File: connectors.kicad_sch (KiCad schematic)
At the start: 4 parts, among them J1 UPT-08-01-01-L-RA, J2 UPT-08-01-01-L-RA, J3 Screw_Terminal_01x02, J4 Conn_01x06

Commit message: Minor fixes
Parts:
- removed J1, J2: UPT-08-01-01-L-RA, UPT080101LRA, symbol 8pin_good:UPT-08-01-01-L-RA
- added J1, J2: UPT-08-01-01-L-RA, UPT080101LRA, symbol UPT-08-01-01-L-RA:UPT-08-01-01-L-RA
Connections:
- net OUT1_0: now also J2.C1, J2.C2, J2.C3, J2.C4, J2.C5, J2.C6
- net OUT1_1: now also J2.B1, J2.B2, J2.B3, J2.B4, J2.B5, J2.B6
- net OUT1_2: now also J2.A1, J2.A2, J2.A3, J2.A4, J2.A5, J2.A6
- net OUT1_3: now also J2.D1, J2.D2, J2.D3, J2.D4, J2.D5, J2.D6
- net OUT2_0: now also J2.H1, J2.H2, J2.H3, J2.H4, J2.H5, J2.H6
- net OUT2_1: now also J2.G1, J2.G2, J2.G3, J2.G4, J2.G5, J2.G6
- net OUT2_2: now also J2.F1, J2.F2, J2.F3, J2.F4, J2.F5, J2.F6
- net OUT2_3: now also J2.E1, J2.E2, J2.E3, J2.E4, J2.E5, J2.E6
- net OUT3_0: now also J1.D1, J1.D2, J1.D3, J1.D4, J1.D5, J1.D6
- net OUT3_1: now also J1.C1, J1.C2, J1.C3, J1.C4, J1.C5, J1.C6
- net OUT3_2: now also J1.B1, J1.B2, J1.B3, J1.B4, J1.B5, J1.B6
- net OUT3_3: now also J1.A1, J1.A2, J1.A3, J1.A4, J1.A5, J1.A6
- net OUT4_0: now also J1.H1, J1.H2, J1.H3, J1.H4, J1.H5, J1.H6
- net OUT4_1: now also J1.G1, J1.G2, J1.G3, J1.G4, J1.G5, J1.G6
- net OUT4_2: now also J1.F1, J1.F2, J1.F3, J1.F4, J1.F5, J1.F6
- net OUT4_3: now also J1.E1, J1.E2, J1.E3, J1.E4, J1.E5, J1.E6

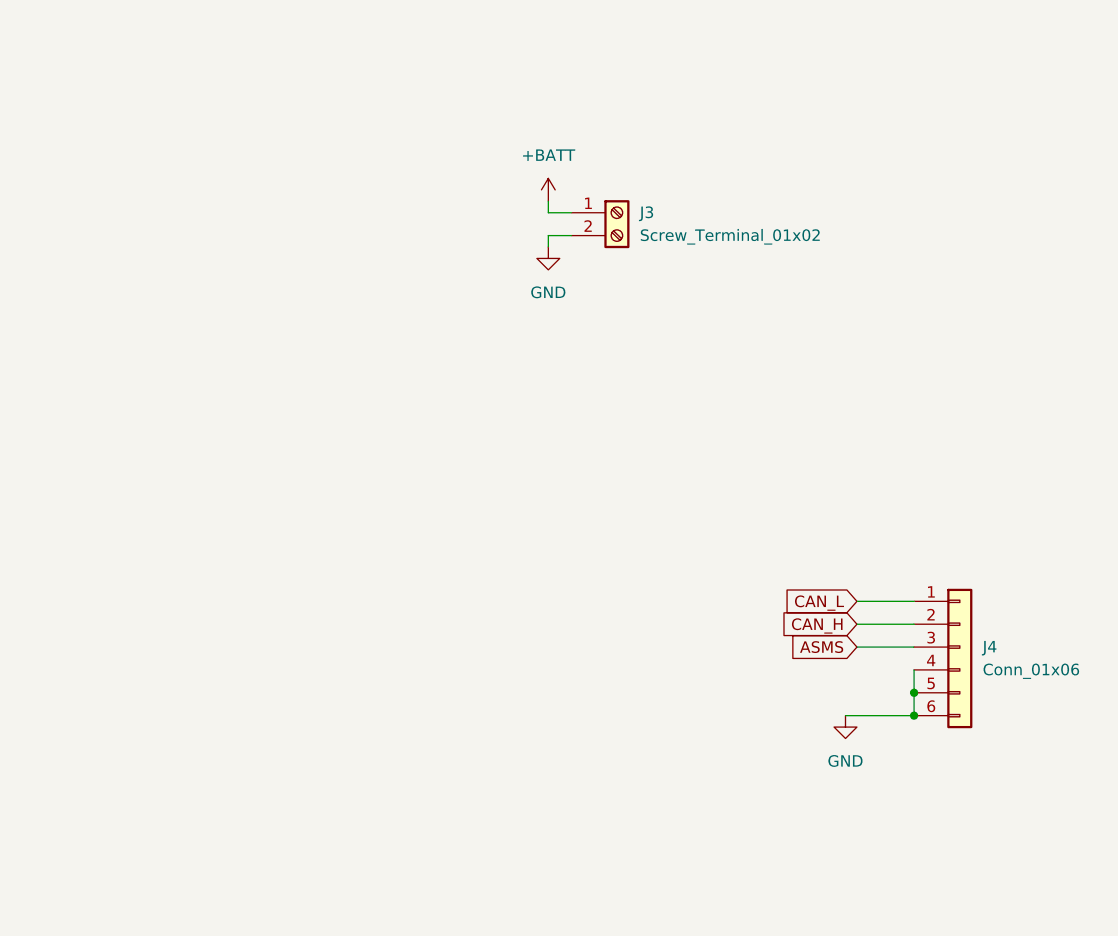
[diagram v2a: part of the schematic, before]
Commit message: Minor changes
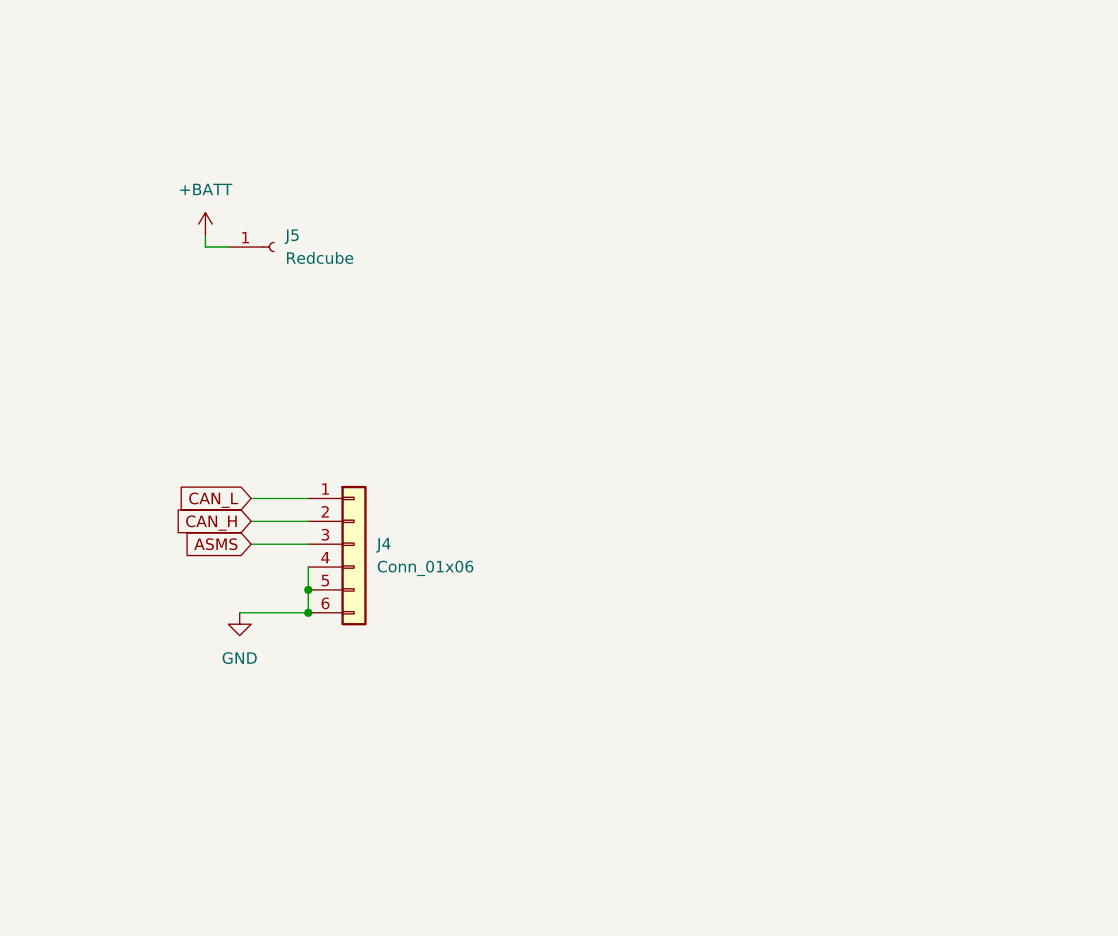
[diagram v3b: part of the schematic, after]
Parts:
- removed J3: Screw_Terminal_01x02, symbol Connector:Screw_Terminal_01x02
- added J5: Redcube, symbol Connector:Conn_01x01_Socket
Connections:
- net +BATT: now also J5.1 (Pin_1)
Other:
- moved on the sheet: J4
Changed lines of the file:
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@@
 	)
 	(junction
-		(at 231.14 105.41)
+		(at 163.83 93.98)
 		(diameter 0)
 		(color 0 0 0 0)
@@
 	)
 	(junction
-		(at 231.14 107.95)
+		(at 163.83 96.52)
 		(diameter 0)
 		(color 0 0 0 0)
@@
 	(wire
 		(pts
-			(xy 224.79 97.79) (xy 231.14 97.79)
+			(xy 157.48 86.36) (xy 163.83 86.36)
 		)
 		(stroke
@@
 	(wire
 		(pts
-			(xy 190.5 54.61) (xy 190.5 55.88)
-		)
-		(stroke
-			(width 0)
-			(type default)
-		)
-	)
-	(wire
-		(pts
-			(xy 224.79 95.25) (xy 231.14 95.25)
+			(xy 157.48 83.82) (xy 163.83 83.82)
 		)
 		(stroke
@@
 	(wire
 		(pts
-			(xy 193.04 52.07) (xy 190.5 52.07)
-		)
-		(stroke
-			(width 0)
-			(type default)
-		)
-	)
-	(wire
-		(pts
 			(xy 95.25 166.37) (xy 95.25 167.64)
 		)
@@
 	(wire
 		(pts
-			(xy 231.14 102.87) (xy 231.14 105.41)
-		)
-		(stroke
-			(width 0)
-			(type default)
-		)
-	)
-	(wire
-		(pts
-			(xy 231.14 105.41) (xy 231.14 107.95)
+			(xy 163.83 91.44) (xy 163.83 93.98)
+		)
+		(stroke
+			(width 0)
+			(type default)
+		)
+	)
+	(wire
+		(pts
+			(xy 163.83 93.98) (xy 163.83 96.52)
 		)
 		(stroke
@@
 	(wire
 		(pts
-			(xy 224.79 100.33) (xy 231.14 100.33)
+			(xy 157.48 88.9) (xy 163.83 88.9)
 		)
 		(stroke
@@
 	(wire
 		(pts
-			(xy 193.04 54.61) (xy 190.5 54.61)
-		)
-		(stroke
-			(width 0)
-			(type default)
-		)
-	)
-	(wire
-		(pts
 			(xy 95.25 49.53) (xy 95.25 52.07)
 		)
@@
 	(wire
 		(pts
-			(xy 190.5 52.07) (xy 190.5 50.8)
+			(xy 152.4 55.88) (xy 152.4 54.61)
 		)
 		(stroke
@@
 	(wire
 		(pts
+			(xy 152.4 55.88) (xy 154.94 55.88)
+		)
+		(stroke
+			(width 0)
+			(type default)
+		)
+	)
+	(wire
+		(pts
 			(xy 95.25 72.39) (xy 95.25 74.93)
 		)
@@
 	(wire
 		(pts
-			(xy 223.52 107.95) (xy 231.14 107.95)
+			(xy 156.21 96.52) (xy 163.83 96.52)
 		)
 		(stroke
@@
 	(global_label "CAN_L"
 		(shape input)
-		(at 224.79 95.25 180)
+		(at 157.48 83.82 180)
 		(fields_autoplaced yes)
 		(effects
@@
 		)
 		(property "Intersheetrefs" "${INTERSHEET_REFS}"
-			(at 216.12 95.25 0)
+			(at 148.81 83.82 0)
 			(effects
 				(font
@@
 	(global_label "ASMS"
 		(shape input)
-		(at 224.79 100.33 180)
+		(at 157.48 88.9 180)
 		(fields_autoplaced yes)
 		(effects
@@
 		)
 		(property "Intersheetrefs" "${INTERSHEET_REFS}"
-			(at 216.8458 100.33 0)
+			(at 149.5358 88.9 0)
 			(effects
 				(font
@@
 	(global_label "CAN_H"
 		(shape input)
-		(at 224.79 97.79 180)
+		(at 157.48 86.36 180)
 		(fields_autoplaced yes)
 		(effects
@@
 		)
 		(property "Intersheetrefs" "${INTERSHEET_REFS}"
-			(at 215.8176 97.79 0)
+			(at 148.5076 86.36 0)
 			(effects
 				(font
@@
 	(symbol
 		(lib_id "power:+BATT")
-		(at 190.5 50.8 0)
+		(at 152.4 54.61 0)
 		(unit 1)
 		(exclude_from_sim no)
@@
 		(fields_autoplaced yes)
 		(property "Reference" "#PWR012"
-			(at 190.5 54.61 0)
+			(at 152.4 58.42 0)
 			(effects
 				(font
@@
 		)
 		(property "Value" "+BATT"
-			(at 190.5 45.72 0)
+			(at 152.4 49.53 0)
 			(effects
 				(font
@@
 		)
 		(property "Footprint" ""
-			(at 190.5 50.8 0)
+			(at 152.4 54.61 0)
 			(effects
 				(font
@@
 		)
 		(property "Datasheet" ""
-			(at 190.5 50.8 0)
+			(at 152.4 54.61 0)
 			(effects
 				(font
@@
 		)
 		(property "Description" ""
-			(at 190.5 50.8 0)
+			(at 152.4 54.61 0)
 			(effects
 				(font
@@
 	)
 	(symbol
-		(lib_id "power:GND")
-		(at 190.5 55.88 0)
+		(lib_id "Connector:Conn_01x01_Socket")
+		(at 160.02 55.88 0)
 		(unit 1)
 		(exclude_from_sim no)
@@
 		(dnp no)
 		(fields_autoplaced yes)
-		(property "Reference" "#PWR013"
-			(at 190.5 62.23 0)
-			(effects
-				(font
-					(size 1.27 1.27)
-				)
-				(hide yes)
-			)
-		)
-		(property "Value" "GND"
-			(at 190.5 60.96 0)
-			(effects
-				(font
-					(size 1.27 1.27)
-				)
+		(property "Reference" "J5"
+			(at 161.29 54.6099 0)
+			(effects
+				(font
+					(size 1.27 1.27)
+				)
+				(justify left)
+			)
+		)
+		(property "Value" "Redcube"
+			(at 161.29 57.1499 0)
+			(effects
+				(font
+					(size 1.27 1.27)
+				)
+				(justify left)
 			)
 		)
 		(property "Footprint" ""
-			(at 190.5 55.88 0)
-			(effects
-				(font
-					(size 1.27 1.27)
-				)
-				(hide yes)
-			)
-		)
-		(property "Datasheet" ""
-			(at 190.5 55.88 0)
-			(effects
-				(font
-					(size 1.27 1.27)
-				)
-				(hide yes)
-			)
-		)
-		(property "Description" ""
-			(at 190.5 55.88 0)
+			(at 160.02 55.88 0)
+			(effects
+				(font
+					(size 1.27 1.27)
+				)
+				(hide yes)
+			)
+		)
+		(property "Datasheet" "https://www.we-online.com/components/products/datasheet/7464100.pdf"
+			(at 160.02 55.88 0)
+			(effects
+				(font
+					(size 1.27 1.27)
+				)
+				(hide yes)
+			)
+		)
+		(property "Description" "7464100"
+			(at 160.02 55.88 0)
+			(effects
+				(font
+					(size 1.27 1.27)
+				)
+				(hide yes)
+			)
+		)
+		(property "Mouser" "https://www.mouser.pl/ProductDetail/Wurth-Elektronik/7464100?qs=vHuUswq2%252BszjGOqwiN7d3A%3D%3D"
+			(at 160.02 55.88 0)
 			(effects
 				(font
@@
 		)
 		(instances
-			(project "PUTM_EV_PDMv2_2024"
+			(project ""
 				(path "/b652b05a-4e3d-4ad1-b032-18886abe7d45/75205686-d634-48ae-88b0-38ad9a9bff05"
-					(reference "#PWR013")
+					(reference "J5")
 					(unit 1)
 				)
@@
 	(symbol
 		(lib_id "Connector_Generic:Conn_01x06")
-		(at 236.22 100.33 0)
+		(at 168.91 88.9 0)
 		(unit 1)
 		(exclude_from_sim no)
@@
 		(fields_autoplaced yes)
 		(property "Reference" "J4"
-			(at 238.76 100.33 0)
+			(at 171.45 88.9 0)
 			(effects
 				(font
@@
 		)
 		(property "Value" "Conn_01x06"
-			(at 238.76 102.87 0)
+			(at 171.45 91.44 0)
 			(effects
 				(font
@@
 		)
 		(property "Footprint" "Connector_IDC:IDC-Header_2x03_P2.54mm_Vertical"
-			(at 236.22 100.33 0)
+			(at 168.91 88.9 0)
 			(effects
 				(font
@@
 		)
 		(property "Datasheet" "~"
-			(at 236.22 100.33 0)
+			(at 168.91 88.9 0)
 			(effects
 				(font
@@
 		)
 		(property "Description" ""
-			(at 236.22 100.33 0)
+			(at 168.91 88.9 0)
 			(effects
 				(font
@@
 	(symbol
 		(lib_id "power:GND")
-		(at 223.52 107.95 0)
+		(at 156.21 96.52 0)
 		(unit 1)
 		(exclude_from_sim no)
@@
 		(fields_autoplaced yes)
 		(property "Reference" "#PWR014"
-			(at 223.52 114.3 0)
+			(at 156.21 102.87 0)
 			(effects
 				(font
@@
 		)
 		(property "Value" "GND"
-			(at 223.52 113.03 0)
+			(at 156.21 101.6 0)
 			(effects
 				(font
@@
 		)
 		(property "Footprint" ""
-			(at 223.52 107.95 0)
+			(at 156.21 96.52 0)
 			(effects
 				(font
@@
 		)
 		(property "Datasheet" ""
-			(at 223.52 107.95 0)
+			(at 156.21 96.52 0)
 			(effects
 				(font
@@
 		)
 		(property "Description" ""
-			(at 223.52 107.95 0)
+			(at 156.21 96.52 0)
 			(effects
 				(font
@@
 					(unit 1)
 				)
-			)
-		)
-	)
-	(symbol
-		(lib_id "Connector:Screw_Terminal_01x02")
-		(at 198.12 52.07 0)
-		(unit 1)
-		(exclude_from_sim no)
-		(in_bom yes)
-		(on_board yes)
-		(dnp no)
-		(fields_autoplaced yes)
-		(property "Reference" "J3"
-			(at 200.66 52.0699 0)
-			(effects
-				(font
-					(size 1.27 1.27)
-				)
-				(justify left)
-			)
-		)
-		(property "Value" "Screw_Terminal_01x02"
-			(at 200.66 54.6099 0)
-			(effects
-				(font
-					(size 1.27 1.27)
-				)
-				(justify left)
-			)
-		)
-		(property "Footprint" ""
-			(at 198.12 52.07 0)
-			(effects
-				(font
-					(size 1.27 1.27)
-				)
-				(hide yes)
-			)
-		)
-		(property "Datasheet" "~"
-			(at 198.12 52.07 0)
-			(effects
-				(font
-					(size 1.27 1.27)
-				)
-				(hide yes)
-			)
-		)
-		(property "Description" "Generic screw terminal, single row, 01x02, script generated (kicad-library-utils/schlib/autogen/connector/)"
-			(at 198.12 52.07 0)
-			(effects
-				(font
-					(size 1.27 1.27)
-				)
-				(hide yes)
-			)
-		)
-		(pin "2"
-		)
-		(pin "1"
-		)
-		(instances
-			(project ""
-				(path "/b652b05a-4e3d-4ad1-b032-18886abe7d45/75205686-d634-48ae-88b0-38ad9a9bff05"
-					(reference "J3")
-					(unit 1)
-				)

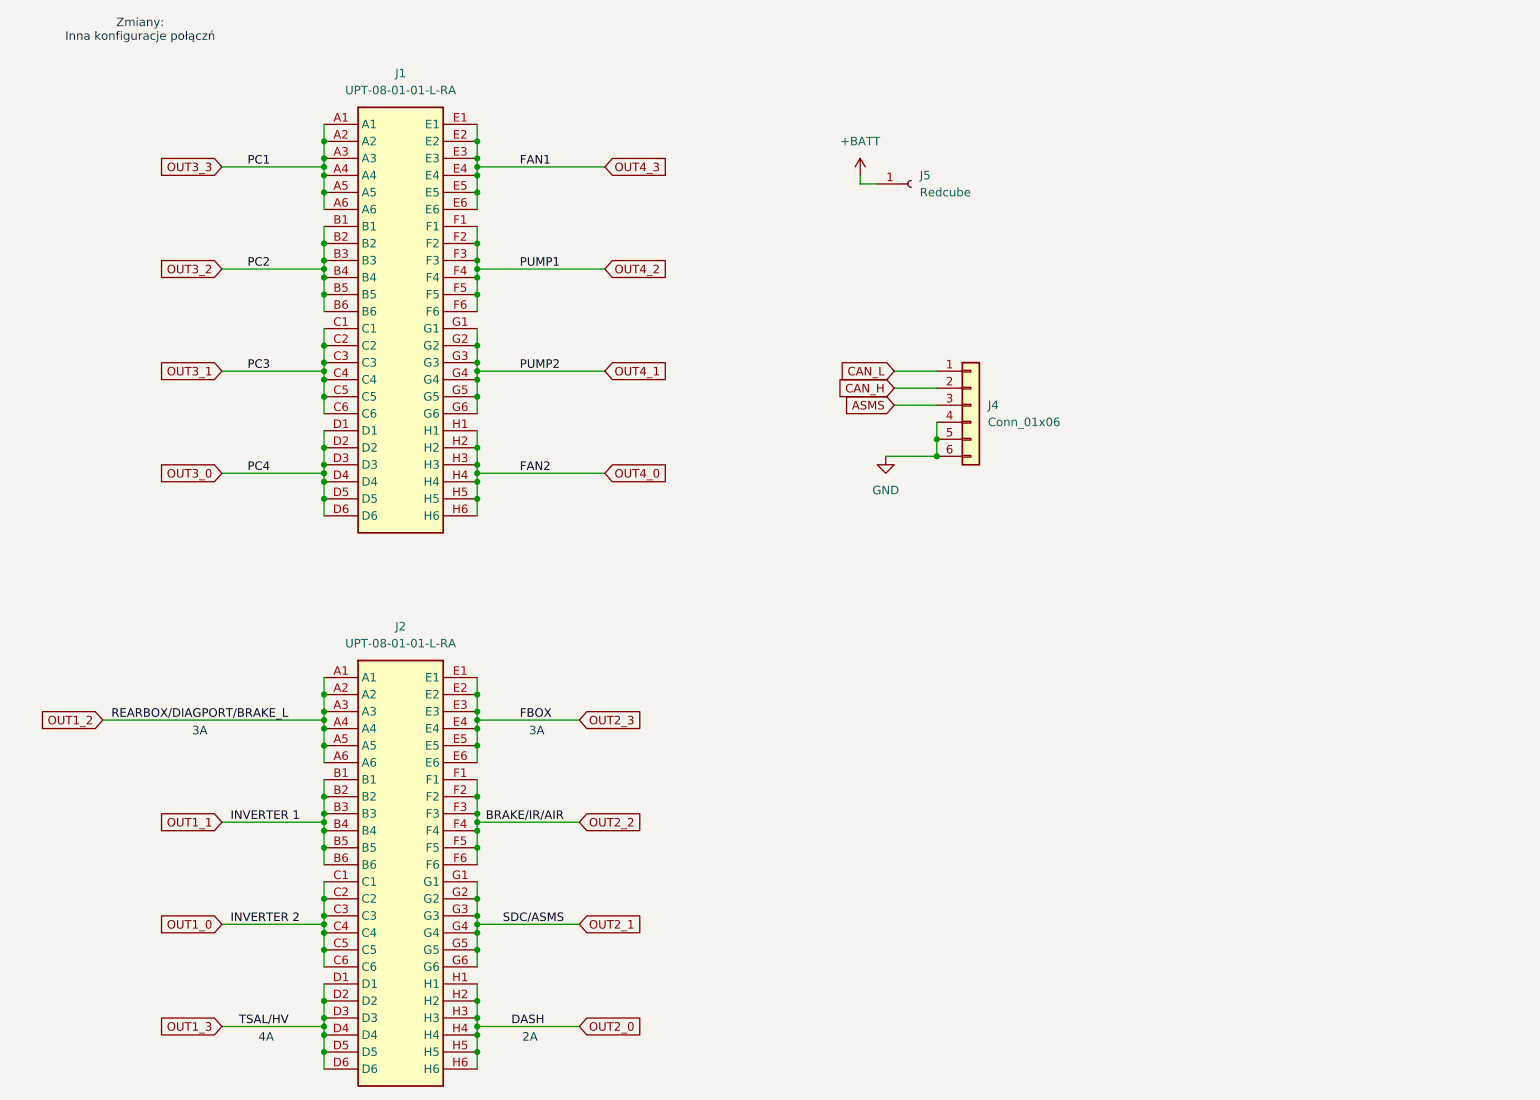
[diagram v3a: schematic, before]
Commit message: Layout done
Added layout
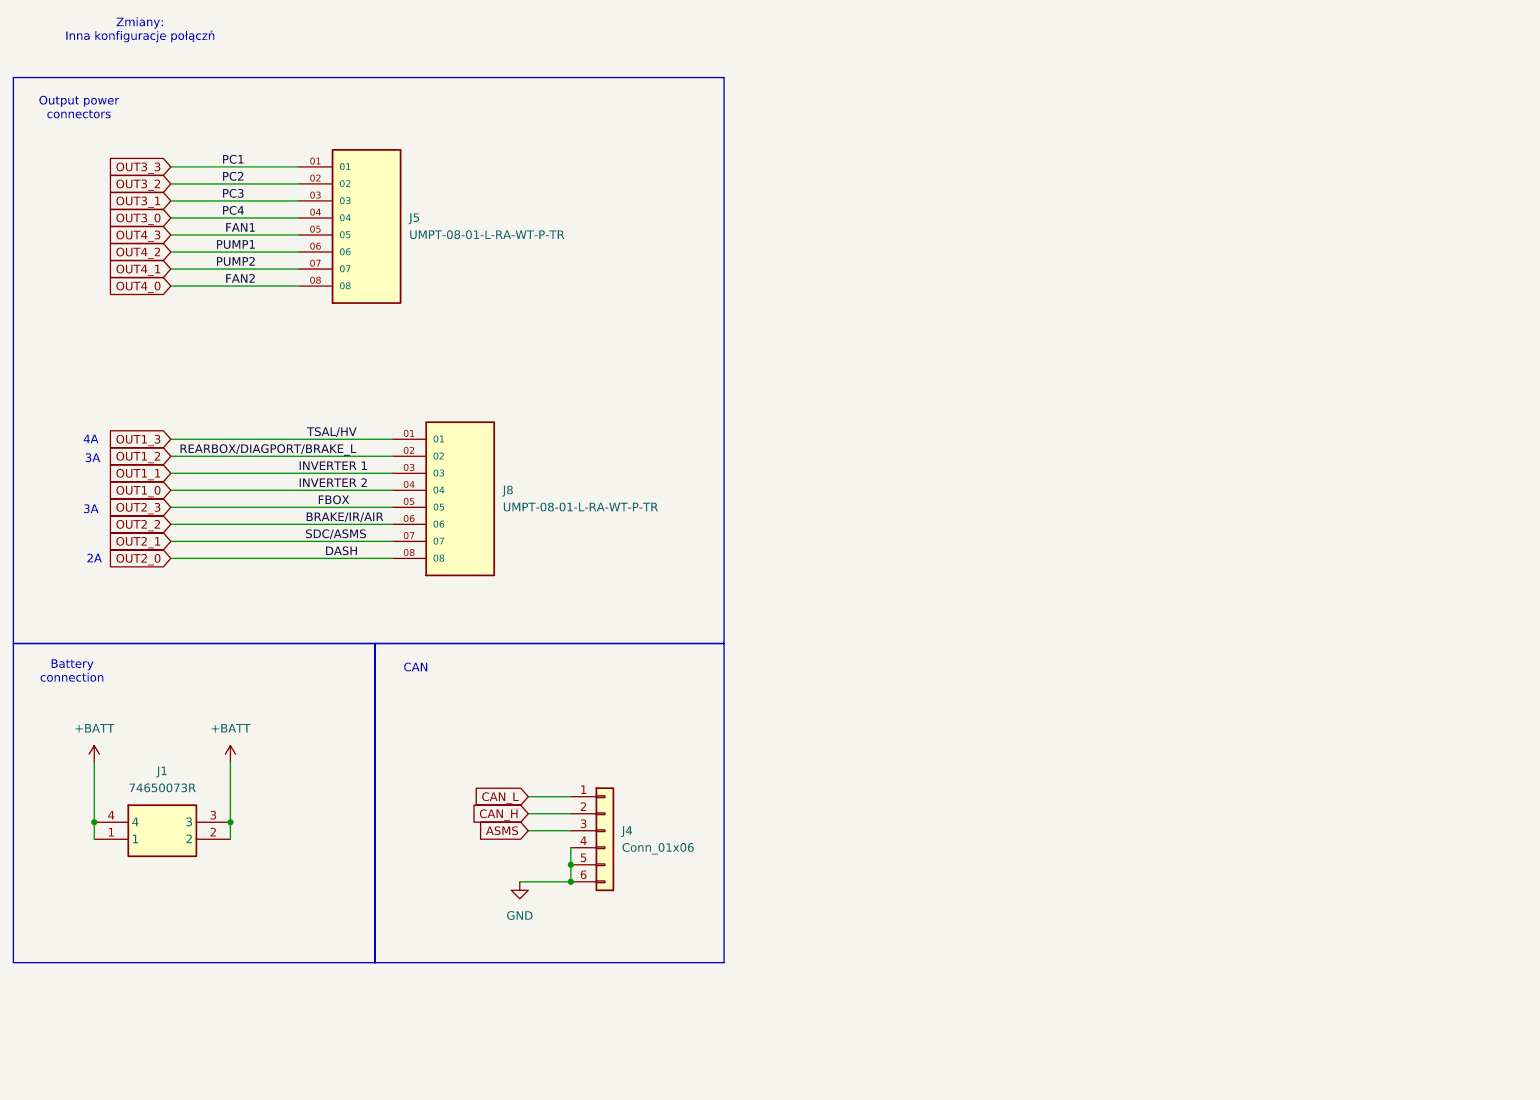
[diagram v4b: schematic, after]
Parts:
- removed J1, J2: UPT-08-01-01-L-RA, UPT080101LRA, symbol UPT-08-01-01-L-RA:UPT-08-01-01-L-RA
- removed J5: Redcube, symbol Connector:Conn_01x01_Socket
- added J1: 74650073R, 74650073R, symbol Redcube_conn:74650073R
- added J5, J8: UMPT-08-01-L-RA-WT-P-TR, UMPT-08-01-L-RA-WT-P-TR:SAMTEC_UMPT-08-01-L-RA-WT-P-TR, symbol UMPT-08-01-L-RA-WT-P-TR:UMPT-08-01-L-RA-WT-P-TR
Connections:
- net +BATT: now also J1.1, J1.2, J1.3, J1.4
- net OUT1_0: now also J8.04
- net OUT1_1: now also J8.03
- net OUT1_2: now also J8.02
- net OUT1_3: now also J8.01
- net OUT2_0: now also J8.08
- net OUT2_1: now also J8.07
- net OUT2_2: now also J8.06
- net OUT2_3: now also J8.05
- net OUT3_0: now also J5.04
- net OUT3_1: now also J5.03
- net OUT3_2: now also J5.02
- net OUT3_3: now also J5.01
- net OUT4_0: now also J5.08
- net OUT4_1: now also J5.07
- net OUT4_2: now also J5.06
- net OUT4_3: now also J5.05
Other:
- note added: "Battery connection"
- note added: "CAN"
- note added: "Output power connectors"
- moved on the sheet: J4
